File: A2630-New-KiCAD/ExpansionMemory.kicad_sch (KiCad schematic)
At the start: 16 parts, among them U102 27C256, U103 27C256, U406 SDRAM_512Mb(32Mx16), U407 SDRAM_512Mb(32Mx16), U408 SDRAM_512Mb(32Mx16), U409 SDRAM_512Mb(32Mx16)

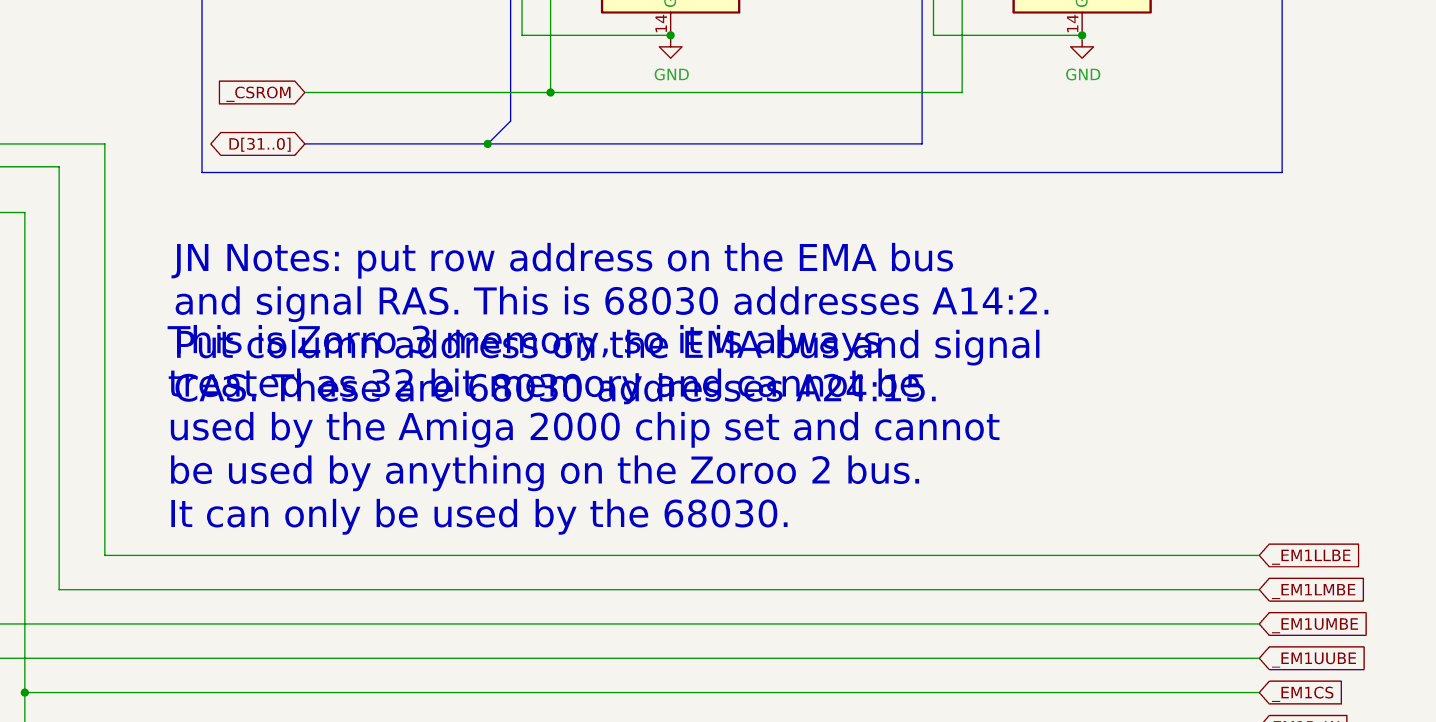
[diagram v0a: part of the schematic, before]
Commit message: Add files via upload
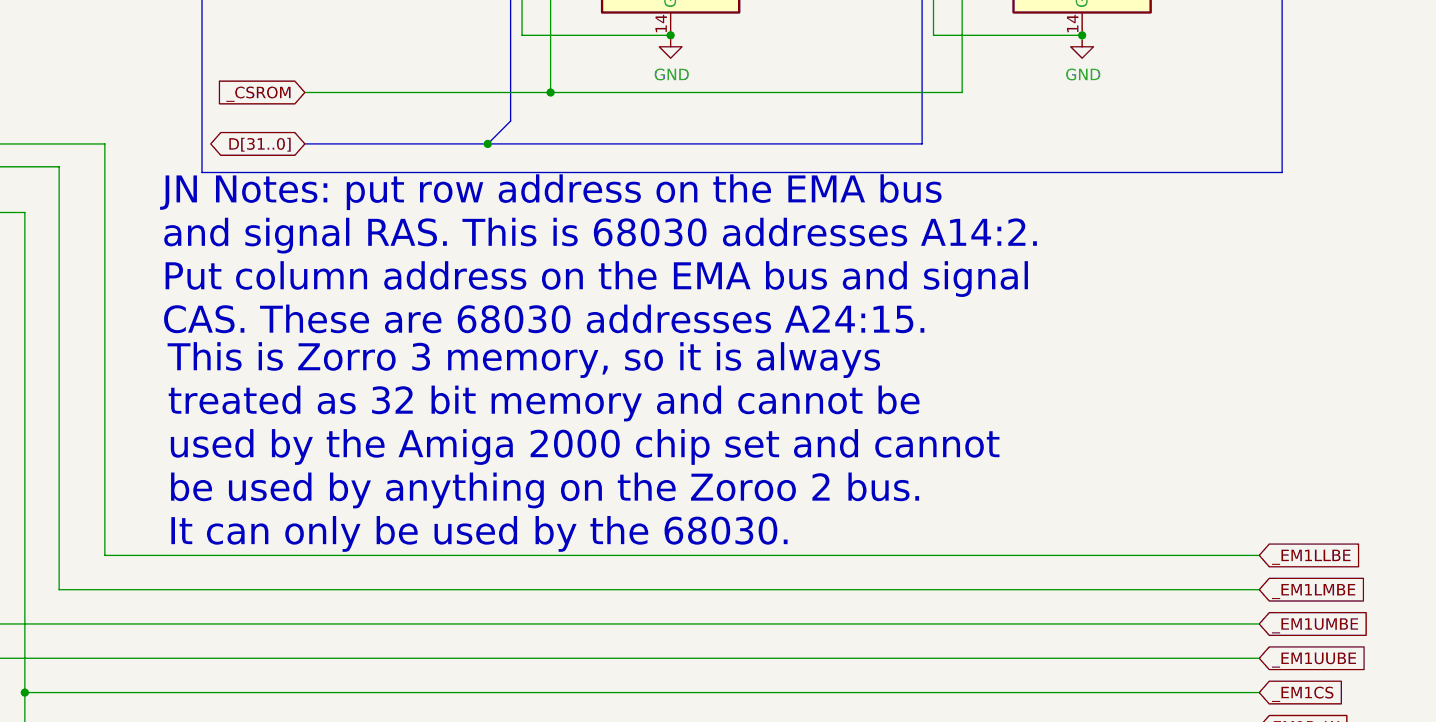
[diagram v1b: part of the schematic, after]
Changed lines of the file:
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@@
   )
   (text "This is Zorro 3 memory, so it is always\ntreated as 32 bit memory and cannot be \nused by the Amiga 2000 chip set and cannot\nbe used by anything on the Zoroo 2 bus.\nIt can only be used by the 68030."
-    (at 274.955 153.67 0)
+    (at 274.955 155.575 0)
     (effects (font (size 3 3)) (justify left bottom))
   )
@@
   )
   (text "JN Notes: put row address on the EMA bus \nand signal RAS. This is 68030 addresses A14:2. \nPut column address on the EMA bus and signal \nCAS. These are 68030 addresses A24:15."
-    (at 275.59 139.7 0)
+    (at 274.32 132.08 0)
     (effects (font (size 2.9972 2.9972)) (justify left bottom))
   )
